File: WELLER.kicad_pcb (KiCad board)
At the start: 2 copper layers, 20 x 100 mm, 59 parts, among them J1 Jack-DC, J2 AudioJack3_Ground_SwitchTR, J3 Conn_02x04_Odd_Even, J4 Conn_01x04_Female, Q1 DMP2018LFK, SW1 SW_Push_SPDT, SW2 SW_Push, SW3 SW_Push, U1 AP1117-33, U2 LTC4440ES6, U3 MCP603-xCH, U4 STM32F103C8Tx

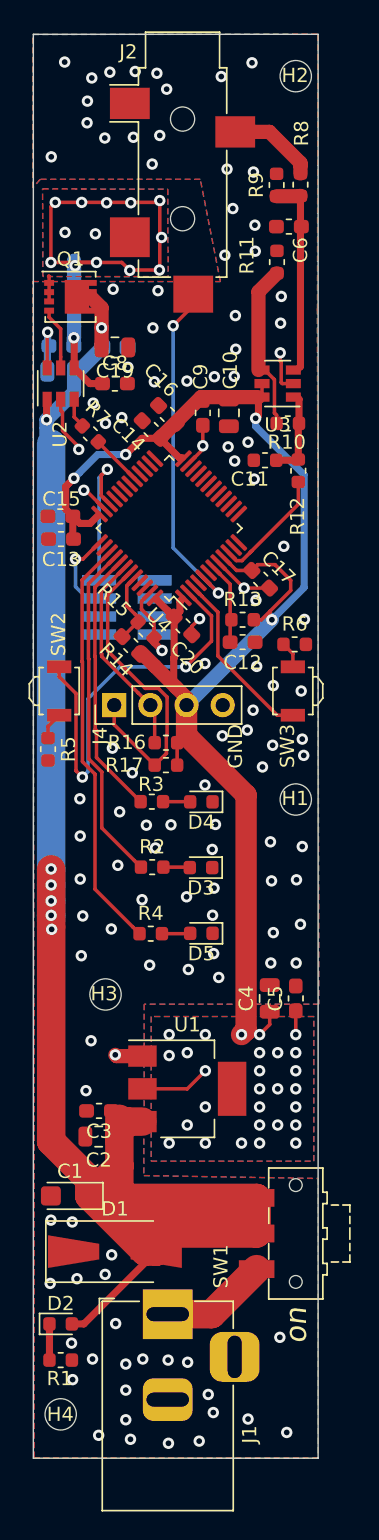
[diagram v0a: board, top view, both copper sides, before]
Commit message: duży update, drc przechodzi
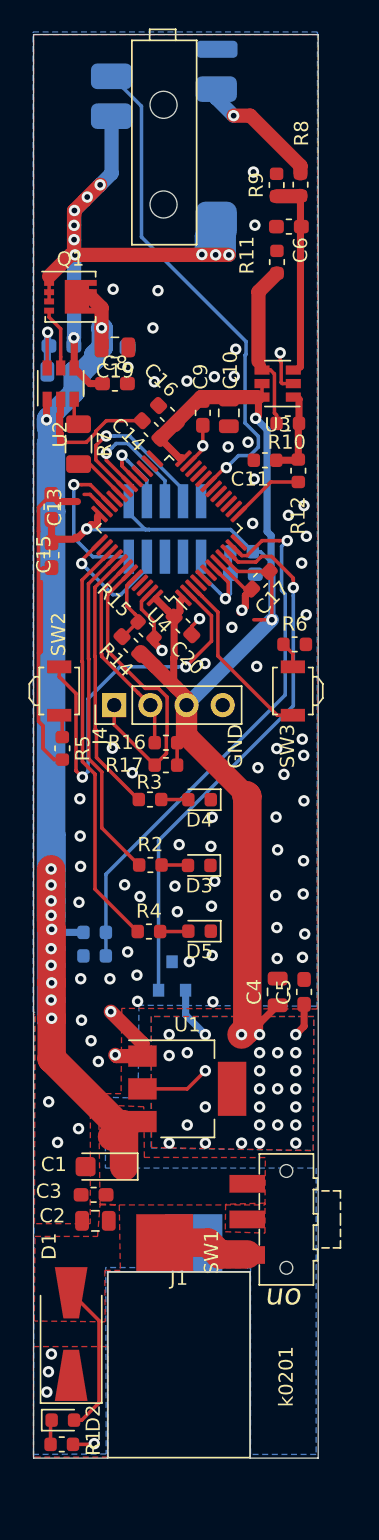
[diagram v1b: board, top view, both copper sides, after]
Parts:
- removed H1, H2, H3, H4: MountingHole, MountingHole:MountingHole_2.2mm_M2
- added R18: 560k, Resistor_SMD:R_0603_1608Metric, B.Cu at (124.3, 88.1)
- added R19: 100k, Resistor_SMD:R_0603_1608Metric, B.Cu at (124.3, 89.7)
- added U5: SM353LT, Package_TO_SOT_SMD:SOT-23, B.Cu at (129.7, 91.1)
- C12, R13: moved to B.Cu
- J1: footprint Connector_BarrelJack:BarrelJack_Horizontal -> symbols:jackDC_cutout
- J2: value AudioJack3_Ground_SwitchTR -> AudioJack3_Ground_SwitchR; footprint Connector_Audio:Jack_3.5mm_CUI_SJ-3524-SMT_Horizontal -> symbols:Jack Audio 1503 20; moved to B.Cu
- J3: value Conn_02x04_Odd_Even -> debug+programing; footprint Connector_PinHeader_1.27mm:PinHeader_2x04_P1.27mm_Vertical_SMD -> Connector_PinHeader_1.27mm:PinHeader_2x05_P1.27mm_Vertical_SMD
- J4: value Conn_01x04_Female -> I2c oled
- R7: footprint Resistor_SMD:R_0603_1608Metric -> Resistor_SMD:R_1206_3216Metric
- moved J2 8.06 mm to (131.4, 25.5), turned to 90 degrees
- moved D2 6.76 mm to (122.1, 122.3)
- moved D1 6.56 mm to (122.7, 116.3), turned to 90 degrees
- moved J3 6.13 mm to (129.2, 59.7), turned to 270 degrees
- moved C2 5.92 mm to (124.4, 108.3)
- moved R1 5.92 mm to (122.0, 124.0)
- moved C3 5.91 mm to (124.2, 106.5)
- moved R13 4.78 mm to (134.6, 61.3)
- moved C12 4.78 mm to (134.7, 62.9)
- moved C1 3.19 mm to (125.0, 104.5)
- moved J1 3.12 mm to (130.2, 111.9), turned to 0 degrees
- moved C13 1.32 mm to (121.3, 61.6), turned to 270 degrees
- moved SW1 1.19 mm to (137.8, 108.2)
- moved R7 1.10 mm to (123.2, 53.8), turned to 270 degrees
- moved R5 1.01 mm to (122.0, 75.1)
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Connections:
- net /tip_driving/12V renamed /stm32/12V
- J2 pad R: /tip_driving/termocouple+ -> /tip_driving/heater
- J2 pad S: GND -> /tip_driving/termocouple+
- J3 pad 1: GND -> /tip_driving/3.3V_analog
- J3 pad 2: /stm32/nRST -> /stm32/SWDIO
- J3 pad 3: GND -> /stm32/usart_rx
- J3 pad 5: GND -> /stm32/usart_tx
- J3 pad 6: /stm32/SWDIO -> (no net)
- J3 pad 7: GND -> /stm32/usart_ck
- J3 pad 8: /stm32/3_3v -> (no net)
- U4 pad 10: /stm32/termocouple -> /stm32/hall_in
- U4 pad 11: Net-(U4-Pad11) -> /stm32/input_divider
- U4 pad 12: Net-(U4-Pad12) -> (no net)
- U4 pad 13: Net-(U4-Pad13) -> /stm32/termocouple
- U4 pad 14: Net-(U4-Pad14) -> (no net)
- U4 pad 15: Net-(U4-Pad15) -> (no net)
- U4 pad 16: Net-(U4-Pad16) -> (no net)
- U4 pad 17: Net-(U4-Pad17) -> (no net)
- U4 pad 18: Net-(U4-Pad18) -> (no net)
- U4 pad 19: Net-(U4-Pad19) -> /stm32/weller_con1
- U4 pad 20: Net-(U4-Pad20) -> (no net)
- U4 pad 21: Net-(U4-Pad21) -> (no net)
- U4 pad 22: Net-(U4-Pad22) -> (no net)
- U4 pad 25: Net-(U4-Pad25) -> (no net)
- U4 pad 26: Net-(U4-Pad26) -> (no net)
- U4 pad 27: Net-(U4-Pad27) -> (no net)
- U4 pad 28: Net-(U4-Pad28) -> (no net)
- U4 pad 29: /tip_driving/HeaterDrivePWM -> /stm32/usart_rx
- U4 pad 30: Net-(U4-Pad30) -> /stm32/usart_tx
- U4 pad 31: Net-(U4-Pad31) -> /stm32/usart_ck
- U4 pad 32: Net-(U4-Pad32) -> /tip_driving/HeaterDrivePWM
- U4 pad 33: Net-(U4-Pad33) -> (no net)
- U4 pad 38: Net-(U4-Pad38) -> (no net)
- U4 pad 4: Net-(U4-Pad4) -> (no net)
- U4 pad 45: Net-(U4-Pad45) -> (no net)
- U4 pad 46: Net-(U4-Pad46) -> (no net)
- U4 pad 5: /stm32/weller_con1 -> (no net)
- U4 pad 6: Net-(U4-Pad6) -> (no net)
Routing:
- net GND: track 25.9 -> 65.3 mm, vias 121 -> 78
- net /stm32/input_divider: track 0.00 -> 39.1 mm, vias 0 -> 1
- net /stm32/hall_in: track 0.00 -> 38.5 mm, vias 0 -> 1
- net /stm32/12V: track 132.7 -> 104.2 mm, vias 7 -> 12
- net /stm32/usart_ck: track 0.00 -> 12.7 mm, vias 0 -> 1
- net /tip_driving/heater: track 38.4 -> 50.7 mm, vias 14 -> 10
- net /tip_driving/3.3V_analog: track 113.7 -> 125.3 mm, vias 32 -> 31
- net /stm32/weller_con1: track 24.4 -> 34.9 mm, vias 2 -> 1
- net /stm32/usart_tx: track 0.00 -> 9.75 mm, vias 0 -> 1
- net /stm32/usart_rx: track 0.00 -> 6.02 mm, vias 0 -> 1
- net /stm32/nRST: track 5.72 -> 9.78 mm, vias 0 -> 1
- net /stm32/termocouple: track 8.49 -> 5.11 mm
- net /stm32/SWCLK: track 6.11 -> 9.07 mm
- net /tip_driving/termocouple+: track 6.22 -> 9.06 mm, vias 0 -> 1
- net Net-(J1-Pad1): track 7.55 -> 6.14 mm
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- added copper zone on F.Cu, net /stm32/12V
- removed copper zone on B.Cu, net /tip_driving/heater
- removed copper zone on F.Cu, net /tip_driving/heater
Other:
- outline, holes or cut-outs redrawn
- board text added: "Weller_RT_tip_solder_v1 05.2019"
- board text removed: "Weller_RT_tip_solder 05.2019"
